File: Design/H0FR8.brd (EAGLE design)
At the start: 34.6 x 30 mm, 46 parts, among them P1 HEXABIT_17.32_NO_P6, Q1 MMBT3904LT1, U1 STM32G0B1CEU6N, U2 T2035H-6GD2PAK_T2550_STM-M, U3 VOT8121AM-VT, U4 TLP184_GR-TPL,SE, X1 XTALL_CSTCE8M00G52

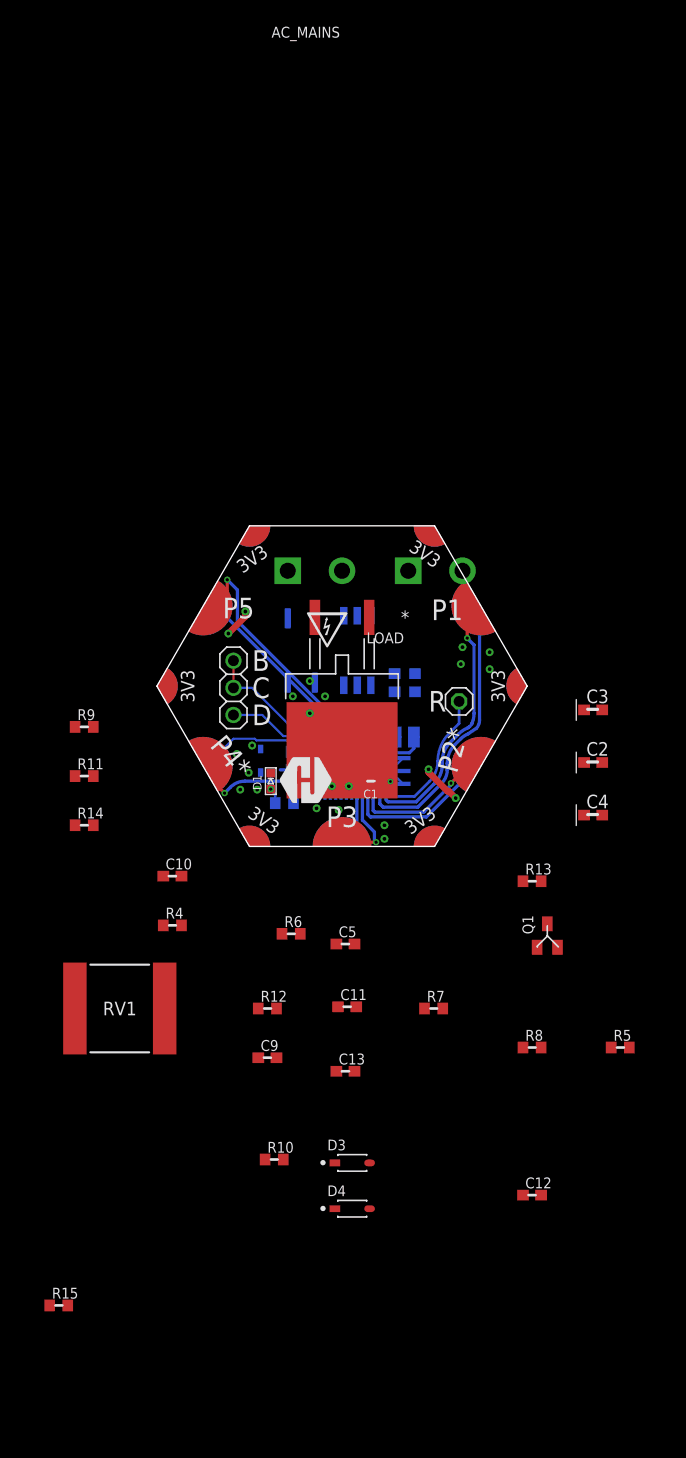
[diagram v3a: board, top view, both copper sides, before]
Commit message: Intial Layout Design
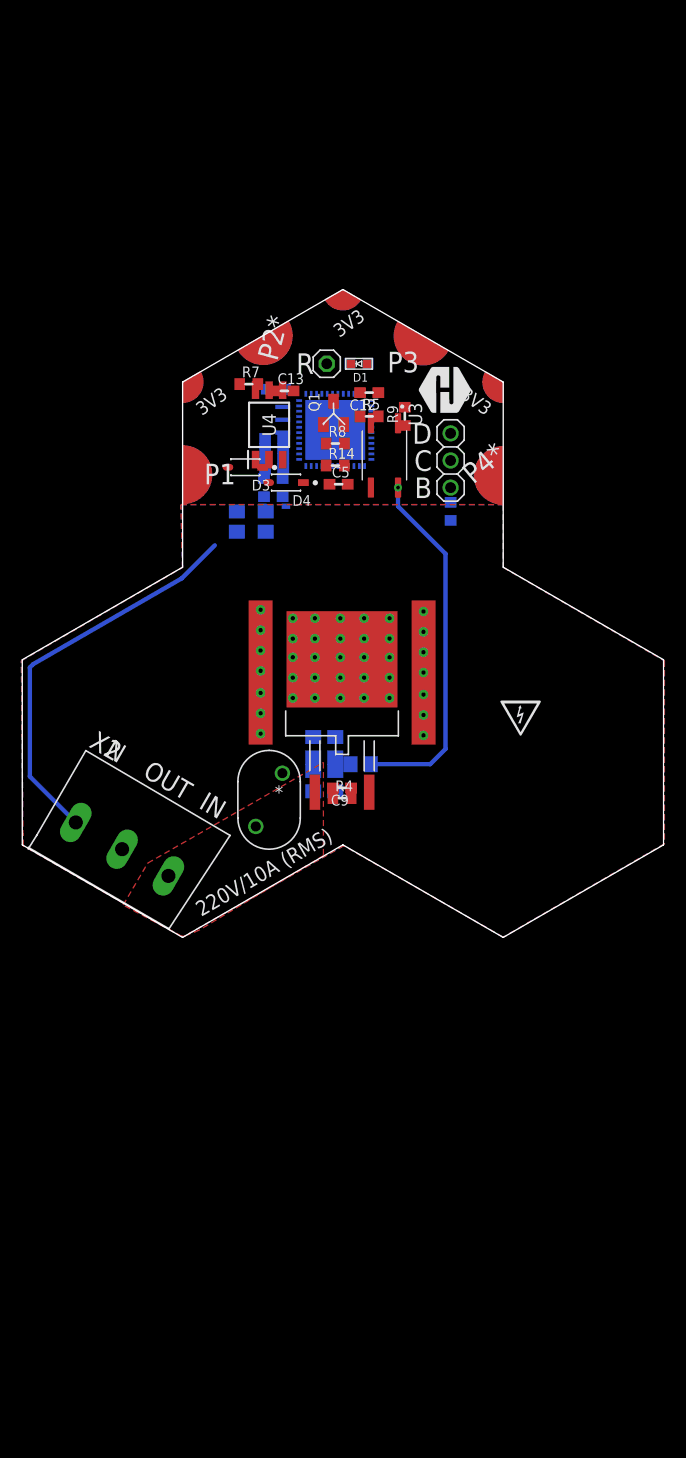
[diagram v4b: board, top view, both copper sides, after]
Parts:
- removed AC_MAINS, LOAD: (no value), HEXABITZ_CONNECTION_PARTS:1546111-2
- removed C4: 4.7uF, HEXABITZ_RCLS:C-0603-POL
- removed C6: 100nF, HEXABITZ_RCLS:C-0603
- removed P1: HEXABIT_17.32_NO_P6, hexabitz_connectors:HEXABIT_17.32_NO_P6
- removed R15: 100k, HEXABITZ_RCLS:R-0603
- removed RV1: MOVS4032V275, HEXABITZ_RCLS:MOVS4032V275
- added U$1: HEXABIT_17.32_X3_NO_P1_P2_P3_P4_P5_P6_P11_P12, hexabitz_connectors:HEXABIT_17.32_X3_NO_P1_P2_P3_P4_P5_P6_P11_P12
- added U$2: FK244D2PAK, HEXABITZ_OTHER_PARTS:FK244D2PAK
- added U5: V275LA4P, HEXABITZ_RCLS:LA_07MM_LOW_LTF
- added X2: (no value), HEXABITZ_CONNECTION_PARTS:AK300/3
- C10, C11: device HEXABITZ_RCLS:C-0603 -> HEXABITZ_RCLS:C-0805
- R10, R11, R12, R13, R6: device HEXABITZ_RCLS:R-0603 -> HEXABITZ_RCLS:R-0805
- U1: value STM32G0B1CEU6N -> STM32G0B1CEU6QFN_B1CEU6_STM-L; device HEXABITZ_ICs:HEXABITZ_ICS_QFN_B1CEU6_STM-L -> HEXABITZ_ICs:QFN_B1CEU6_STM-L
- moved C12 76.6 mm to (2.54, 42.4), turned to 180 degrees
- moved D4 68.2 mm to (-5.24, 34.0), turned to 180 degrees
- moved D3 65.9 mm to (-9.05, 35.4), turned to 180 degrees
- moved C13 63.9 mm to (-5.40, 42.5)
- moved R5 63.6 mm to (2.54, 40.2)
- moved R7 60.9 mm to (-8.73, 43.2)
- moved R10 59.8 mm to (-9.84, 30.3), flipped to the bottom, turned to 270 degrees
- moved R8 59.4 mm to (-0.64, 37.6)
- moved Q1 52.8 mm to (-0.79, 40.5)
- moved C5 43.0 mm to (-0.32, 33.8)
- moved R9 41.8 mm to (5.87, 40.2), turned to 90 degrees
- moved R1 41.7 mm to (1.59, 45.1)
- moved R14 41.0 mm to (-0.64, 35.6)
- moved C2 40.6 mm to (-6.35, 35.2), flipped to the bottom
- moved D1 39.9 mm to (1.59, 45.1), turned to 270 degrees
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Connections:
- removed net AGND: C3.2, C7.2, R3.2, U1.7
- net A2: now also U$2.P$1, U$2.P$2, U5.2, X2.2; no longer LOAD.2, RV1.1
- net AC_MAINS_L: now also C10.2, C11.2, C9.2, R4.1, U2.1, U5.1, X2.3; no longer AC_MAINS.1, LOAD.1
- net AC_MAINS_N: now also X2.1; no longer AC_MAINS.2, C10.2, C11.2, C9.2, R4.1, RV1.2, U2.1
- net GND: now also U$1.PAD_PD12, U$1.PAD_PD17, U$1.PAD_PD19; no longer C4.2, C6.2, P1.PAD_PD10, P1.PAD_PD11, P1.PAD_PD12, P1.PAD_PD7, P1.PAD_PD8, P1.PAD_PD9, R15.2, U1.30
- net N$13: no longer R15.1
- net USART1_RX: now also U$1.PAD_PD8; no longer P1.PAD_PD4
- net USART1_TX: now also U$1.PAD_PU8; no longer P1.PAD_PU4
- net USART2_RX: now also U$1.PAD_PD1; no longer P1.PAD_PD2
- net USART2_TX: now also U$1.PAD_PU1; no longer P1.PAD_PU2
- net USART4_RX: now also U$1.PAD_PD3; no longer P1.PAD_PD1
- net USART4_TX: now also U$1.PAD_PU3; no longer P1.PAD_PU1
- net USART5_RX: no longer P1.PAD_PD5
- net USART5_TX: no longer P1.PAD_PU5
- net USART6_RX: now also U$1.PAD_PD2; no longer P1.PAD_PD3
- net USART6_TX: now also U$1.PAD_PU2; no longer P1.PAD_PU3
- net VDD: now also U$1.PAD_PU12, U$1.PAD_PU17, U$1.PAD_PU19; no longer C4.1, C6.1, P1.PAD_PU10, P1.PAD_PU11, P1.PAD_PU12, P1.PAD_PU7, P1.PAD_PU8, P1.PAD_PU9, U1.31
- net VSSA: now also C3.2, C7.2, R3.2, U1.7
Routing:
- net AC_MAINS_N: track 0.00 -> 37.1 mm
- net N$8: track 0.00 -> 33.9 mm, vias 0 -> 1
- net USART4_RX: track 25.9 -> 0.00 mm
- net USART4_TX: track 25.3 -> 0.00 mm, vias 1 -> 0
- net USART5_TX: track 21.3 -> 0.00 mm, vias 1 -> 0
- net USART5_RX: track 16.0 -> 0.00 mm
- net N$2: track 15.9 -> 0.00 mm, vias 1 -> 0
- net USART2_RX: track 14.2 -> 0.00 mm
- net USART2_TX: track 12.8 -> 0.00 mm, vias 1 -> 0
- net USART1_TX: track 12.1 -> 0.00 mm, vias 1 -> 0
- net CLK: track 11.2 -> 0.00 mm
- net USART1_RX: track 10.9 -> 0.00 mm
- net GND: track 9.81 -> 0.00 mm, vias 23 -> 0
- net USART6_TX: track 8.08 -> 0.00 mm, vias 1 -> 0
- net DATA: track 7.78 -> 0.00 mm
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- added copper zone on layer 1, net A2
- added copper zone on layer 16, net A2
- added copper zone on layer 1, net AC_MAINS_L
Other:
- board size 34.6 x 30 mm -> 60 x 60.6 mm
- board text added: "220V/10A (RMS)"
- board text added: "IN"
- board text added: "N"
- board text added: "OUT"
- board text removed: "600VAC/1.2A"
- board text removed: "P5"
